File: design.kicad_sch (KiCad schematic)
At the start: 26 parts, among them J1 490107670412, J2 TYPE-C-31-M-12, J4 Conn_02x02_Counter_Clockwise, SW3 EN, U1 AP2112K-3.3, U2 TCK107AF,LF, U3 CH340C, U4 TS3USB30RSWR

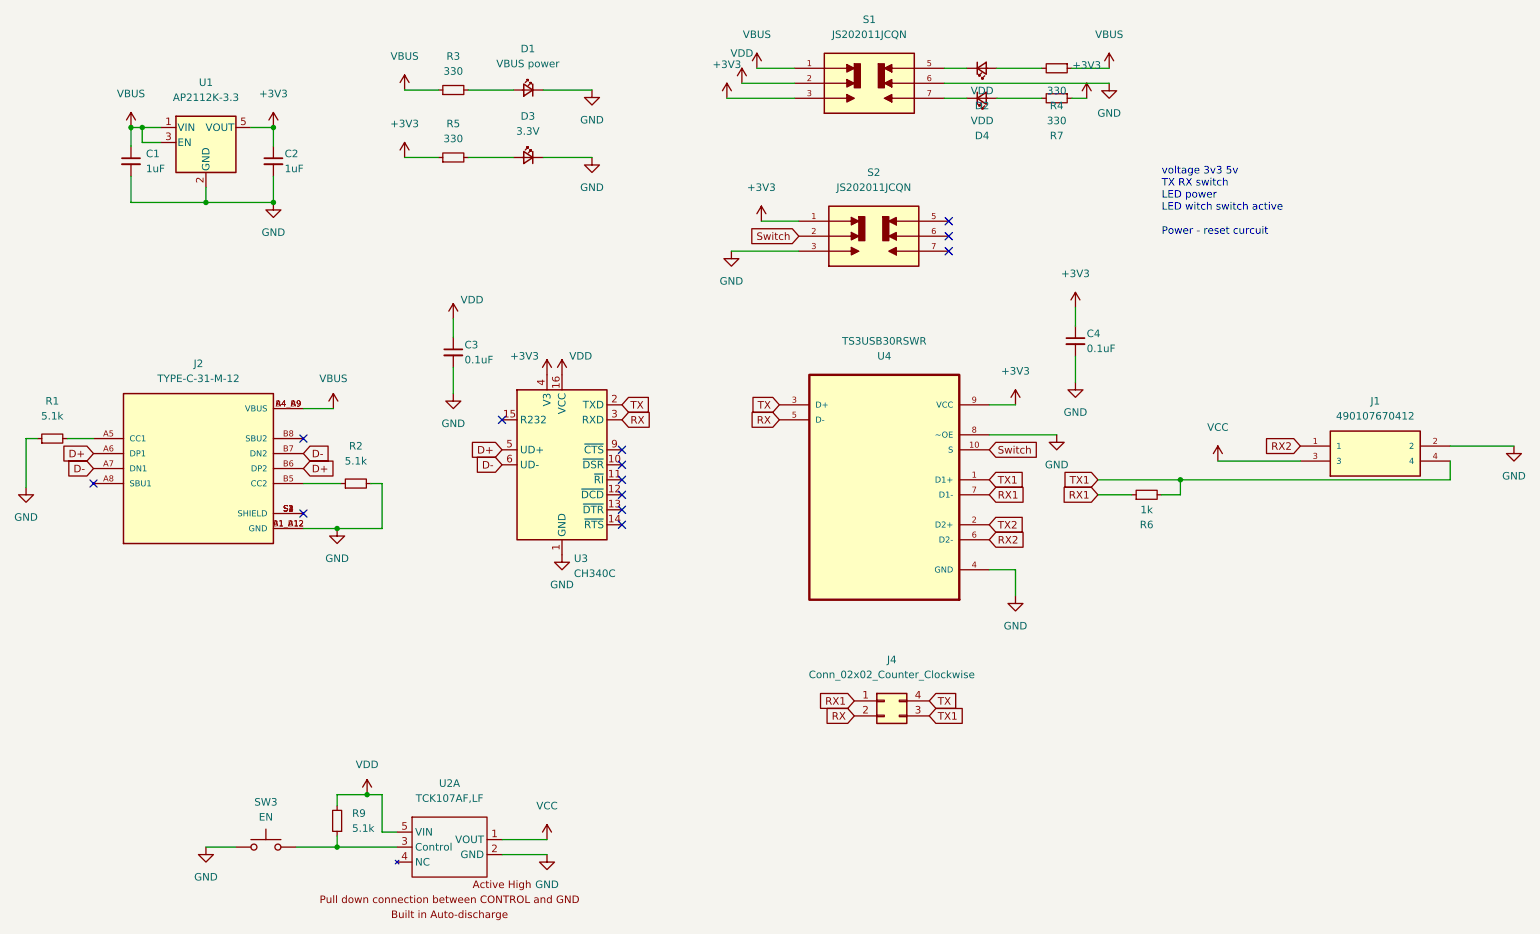
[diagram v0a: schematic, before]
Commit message: update
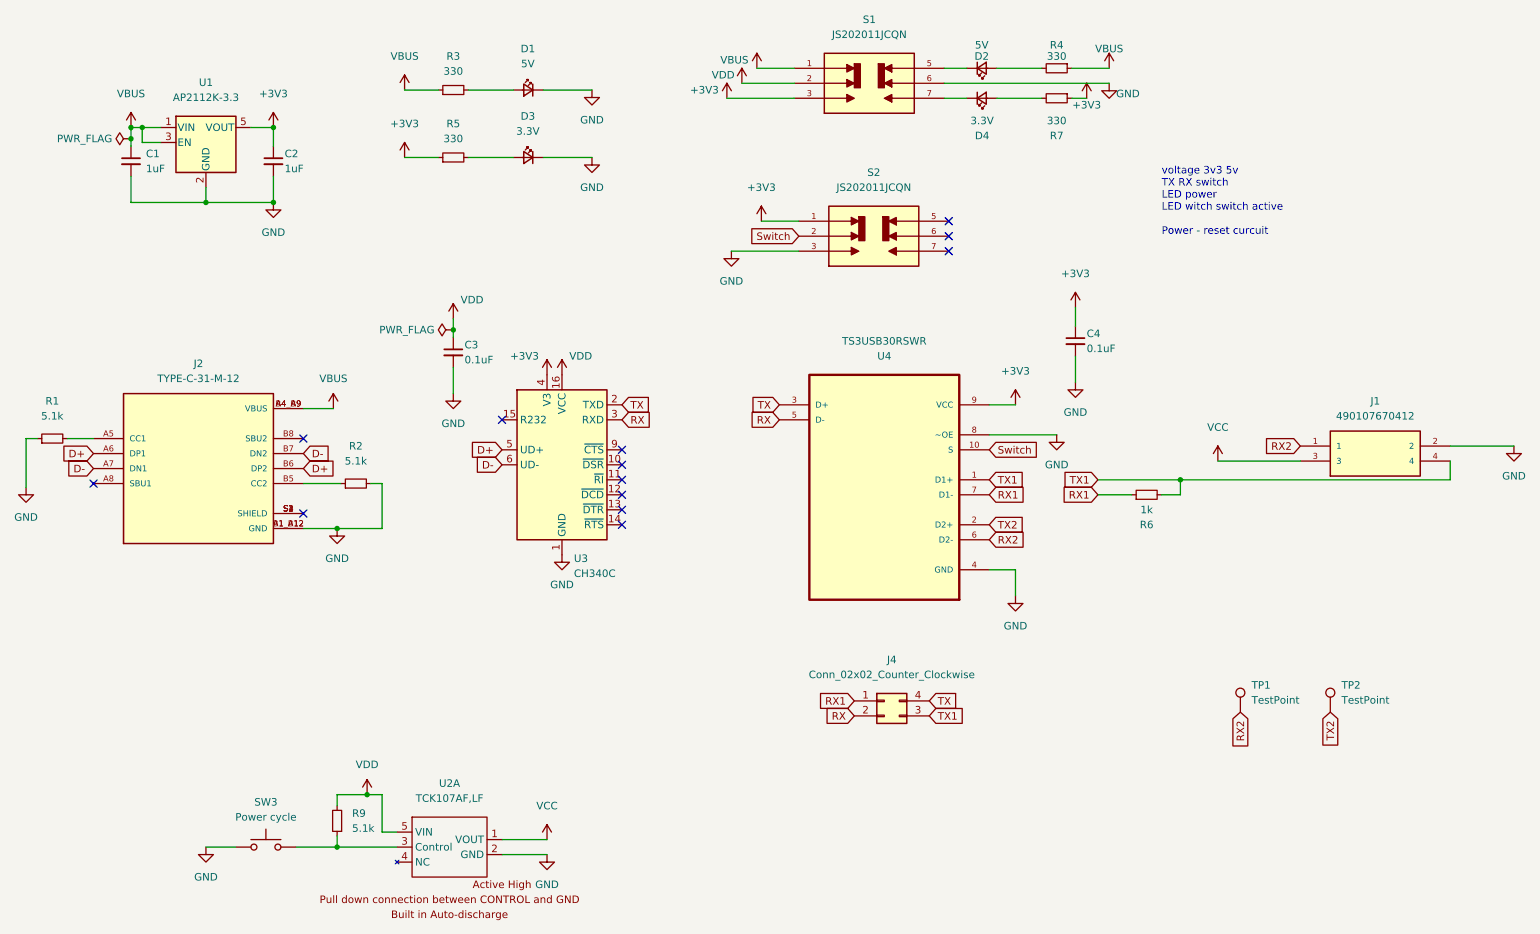
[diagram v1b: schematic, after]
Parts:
- added TP1, TP2: TestPoint, TestPoint:TestPoint_Pad_D2.0mm, symbol Connector:TestPoint
- D1: value VBUS power -> 5V
- D2: value VDD -> 5V
- D4: value VDD -> 3.3V
- SW3: value EN -> Power cycle
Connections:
- net RX2: now also TP1.1
- net TX2: now also TP2.1
